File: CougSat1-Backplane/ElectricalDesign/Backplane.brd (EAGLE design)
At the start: 82.8 x 86 mm, 17 parts, among them J1 CougSat Socket, J10 CougSat Socket, J2 CougSat Socket, J3 CougSat Socket, J4 CougSat Socket, J5 Separation Switch, J6 Separation Switch, J7 CougSat Socket, J8 CougSat Socket, J9 CougSat Socket

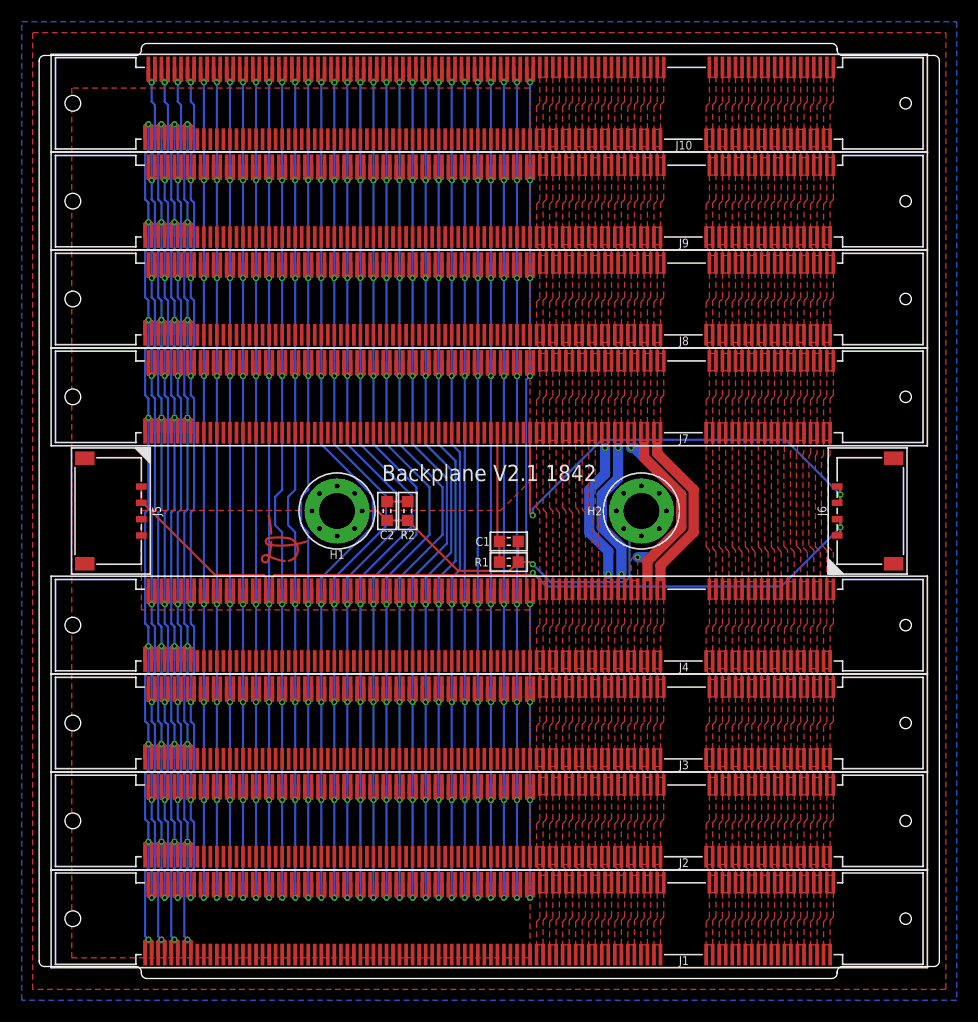
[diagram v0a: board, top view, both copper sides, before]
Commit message: Merge branch 'master' into panel+X
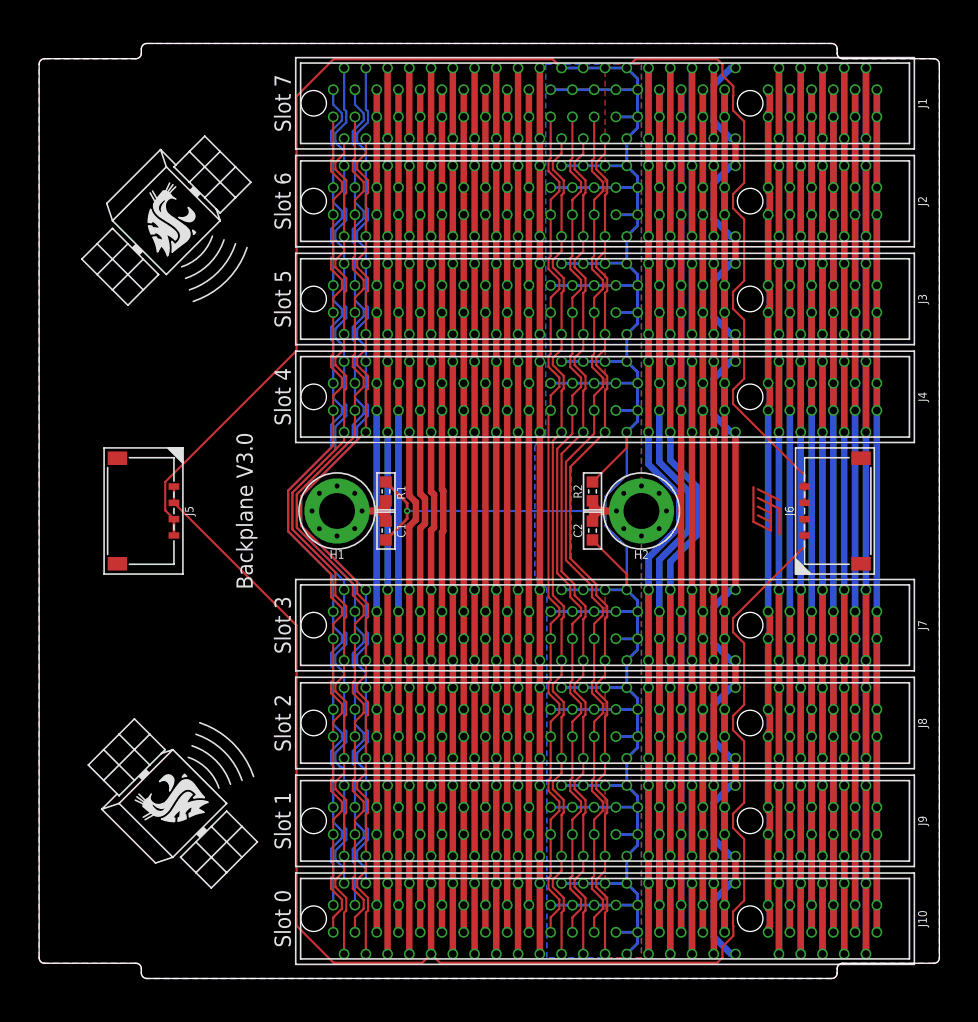
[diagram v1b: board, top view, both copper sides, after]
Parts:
- added LOGO100, LOGO3: Satellite 16mm, CougsInSpace-Aesthetics:CIS-SATELLITE-16
- added LOGO2: SIGNATUREHENDRIK, CougsInSpace-Aesthetics:SIGN-HENDRIK
- J1, J10, J2, J3, J4, J7, J8, J9: device CougsInSpace-Connectors:SODIMM-DDR1 -> CougsInSpace-Connectors:PCIE-8
- LOGO1: value SIGNATUREBRADLEY -> Text; device CougsInSpace-Aesthetics:SIGN-BRADLEY -> CougsInSpace-Aesthetics:CIS-TEXT
- moved J1 78.7 mm to (24.0, 37.5)
- moved J10 78.7 mm to (24.0, -37.5)
- moved J2 61.8 mm to (24.0, 28.5)
- moved J9 61.8 mm to (24.0, -28.5)
- moved J3 45.8 mm to (24.0, 19.5)
- moved J8 45.8 mm to (24.0, -19.5)
- moved J4 31.9 mm to (24.0, 10.5)
- moved J7 31.9 mm to (24.0, -10.5)
- moved C2 19.0 mm to (9.50, -1.80), turned to 270 degrees
- moved R2 17.1 mm to (9.50, 1.80)
- moved R1 13.0 mm to (-9.50, 1.80), turned to 270 degrees
- moved C1 11.3 mm to (-9.50, -1.80), turned to 270 degrees
- moved LOGO1 9.97 mm to (-28.4, 0.10), flipped to the bottom, turned to 90 degrees
- moved J5 3.00 mm to (-29.0, 0.00)
- moved J6 3.00 mm to (29.0, 0.00)
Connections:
- removed net CHASSIS: C1.1, C2.1, H1.1, H1.V1, H1.V2, H1.V3, H1.V4, H1.V5, H1.V6, H1.V7, H1.V8, H2.1, H2.V1, H2.V2, H2.V3, H2.V4, H2.V5, H2.V6, H2.V7, H2.V8, R1.2, R2.2
- removed net GPIO-6: J1.105, J1.107, J10.105, J10.107, J2.105, J2.107, J3.105, J3.107, J4.105, J4.107, J7.105, J7.107, J8.105, J8.107, J9.105, J9.107
- removed net GPIO-7: J1.109, J1.111, J10.109, J10.111, J2.109, J2.111, J3.109, J3.111, J4.109, J4.111, J7.109, J7.111, J8.109, J8.111, J9.109, J9.111
- removed net GPIO-8: J1.113, J1.115, J10.113, J10.115, J2.113, J2.115, J3.113, J3.115, J4.113, J4.115, J7.113, J7.115, J8.113, J8.115, J9.113, J9.115
- removed net GPIO-9: J1.117, J1.119, J10.117, J10.119, J2.117, J2.119, J3.117, J3.119, J4.117, J4.119, J7.117, J7.119, J8.117, J8.119, J9.117, J9.119
- new net CHASSIS1: C1.1, H1.1, H1.V1, H1.V2, H1.V3, H1.V4, H1.V5, H1.V6, H1.V7, H1.V8, R1.2
- new net CHASSIS2: C2.1, H2.1, H2.V1, H2.V2, H2.V3, H2.V4, H2.V5, H2.V6, H2.V7, H2.V8, R2.2
- net BUS_I2C0_IRQ: now also J1.A45, J1.B45, J10.A45, J10.B45, J2.A45, J2.B45, J3.A45, J3.B45, J4.A45, J4.B45, J7.A45, J7.B45, J8.A45, J8.B45, J9.A45, J9.B45; no longer J1.181, J1.183, J10.181, J10.183, J2.181, J2.183, J3.181, J3.183, J4.181, J4.183, J7.181, J7.183, J8.181, J8.183, J9.181, J9.183
- net BUS_I2C0_SCL: now also J1.A44, J1.B44, J10.A44, J10.B44, J2.A44, J2.B44, J3.A44, J3.B44, J4.A44, J4.B44, J7.A44, J7.B44, J8.A44, J8.B44, J9.A44, J9.B44; no longer J1.177, J1.179, J10.177, J10.179, J2.177, J2.179, J3.177, J3.179, J4.177, J4.179, J7.177, J7.179, J8.177, J8.179, J9.177, J9.179
- net BUS_I2C0_SDA: now also J1.A43, J1.B43, J10.A43, J10.B43, J2.A43, J2.B43, J3.A43, J3.B43, J4.A43, J4.B43, J7.A43, J7.B43, J8.A43, J8.B43, J9.A43, J9.B43; no longer J1.173, J1.175, J10.173, J10.175, J2.173, J2.175, J3.173, J3.175, J4.173, J4.175, J7.173, J7.175, J8.173, J8.175, J9.173, J9.175
- net BUS_I2C1_IRQ: now also J1.A32, J1.B32, J10.A32, J10.B32, J2.A32, J2.B32, J3.A32, J3.B32, J4.A32, J4.B32, J7.A32, J7.B32, J8.A32, J8.B32, J9.A32, J9.B32; no longer J1.129, J1.131, J10.129, J10.131, J2.129, J2.131, J3.129, J3.131, J4.129, J4.131, J7.129, J7.131, J8.129, J8.131, J9.129, J9.131
- net BUS_I2C1_SCL: now also J1.A31, J1.B31, J10.A31, J10.B31, J2.A31, J2.B31, J3.A31, J3.B31, J4.A31, J4.B31, J7.A31, J7.B31, J8.A31, J8.B31, J9.A31, J9.B31; no longer J1.125, J1.127, J10.125, J10.127, J2.125, J2.127, J3.125, J3.127, J4.125, J4.127, J7.125, J7.127, J8.125, J8.127, J9.125, J9.127
- net BUS_I2C1_SDA: now also J1.A30, J1.B30, J10.A30, J10.B30, J2.A30, J2.B30, J3.A30, J3.B30, J4.A30, J4.B30, J7.A30, J7.B30, J8.A30, J8.B30, J9.A30, J9.B30; no longer J1.121, J1.123, J10.121, J10.123, J2.121, J2.123, J3.121, J3.123, J4.121, J4.123, J7.121, J7.123, J8.121, J8.123, J9.121, J9.123
- net BUS_JTAG_EN-0: now also J1.B46, J10.B46, J2.B46, J3.B46, J4.B46, J7.B46, J8.B46, J9.B46; no longer J1.186, J1.188, J10.186, J10.188, J2.186, J2.188, J3.186, J3.188, J4.186, J4.188, J7.186, J7.188, J8.186, J8.188, J9.186, J9.188
- net BUS_JTAG_EN-1: now also J1.B47, J10.B47, J2.B47, J3.B47, J4.B47, J7.B47, J8.B47, J9.B47; no longer J1.190, J1.192, J10.190, J10.192, J2.190, J2.192, J3.190, J3.192, J4.190, J4.192, J7.190, J7.192, J8.190, J8.192, J9.190, J9.192
- net BUS_JTAG_EN-2: now also J1.B48, J10.B48, J2.B48, J3.B48, J4.B48, J7.B48, J8.B48, J9.B48; no longer J1.194, J1.196, J10.194, J10.196, J2.194, J2.196, J3.194, J3.196, J4.194, J4.196, J7.194, J7.196, J8.194, J8.196, J9.194, J9.196
- net BUS_JTAG_EN-3: now also J1.B49, J10.B49, J2.B49, J3.B49, J4.B49, J7.B49, J8.B49, J9.B49; no longer J1.198, J1.200, J10.198, J10.200, J2.198, J2.200, J3.198, J3.200, J4.198, J4.200, J7.198, J7.200, J8.198, J8.200, J9.198, J9.200
- net BUS_JTAG_TCK: now also J1.A46, J10.A46, J2.A46, J3.A46, J4.A46, J7.A46, J8.A46, J9.A46; no longer J1.185, J1.187, J10.185, J10.187, J2.185, J2.187, J3.185, J3.187, J4.185, J4.187, J7.185, J7.187, J8.185, J8.187, J9.185, J9.187
- net BUS_JTAG_TDI: now also J1.A47, J10.A47, J2.A47, J3.A47, J4.A47, J7.A47, J8.A47, J9.A47; no longer J1.189, J1.191, J10.189, J10.191, J2.189, J2.191, J3.189, J3.191, J4.189, J4.191, J7.189, J7.191, J8.189, J8.191, J9.189, J9.191
- net BUS_JTAG_TDO: now also J1.A48, J10.A48, J2.A48, J3.A48, J4.A48, J7.A48, J8.A48, J9.A48; no longer J1.193, J1.195, J10.193, J10.195, J2.193, J2.195, J3.193, J3.195, J4.193, J4.195, J7.193, J7.195, J8.193, J8.195, J9.193, J9.195
- net BUS_JTAG_TMS: now also J1.A49, J10.A49, J2.A49, J3.A49, J4.A49, J7.A49, J8.A49, J9.A49; no longer J1.197, J1.199, J10.197, J10.199, J2.197, J2.199, J3.197, J3.199, J4.197, J4.199, J7.197, J7.199, J8.197, J8.199, J9.197, J9.199
- net BUS_SPI_MISO: now also J1.A38, J1.B38, J10.A38, J10.B38, J2.A38, J2.B38, J3.A38, J3.B38, J4.A38, J4.B38, J7.A38, J7.B38, J8.A38, J8.B38, J9.A38, J9.B38; no longer J1.153, J1.155, J10.153, J10.155, J2.153, J2.155, J3.153, J3.155, J4.153, J4.155, J7.153, J7.155, J8.153, J8.155, J9.153, J9.155
- net BUS_SPI_MOSI: now also J1.A39, J1.B39, J10.A39, J10.B39, J2.A39, J2.B39, J3.A39, J3.B39, J4.A39, J4.B39, J7.A39, J7.B39, J8.A39, J8.B39, J9.A39, J9.B39; no longer J1.157, J1.159, J10.157, J10.159, J2.157, J2.159, J3.157, J3.159, J4.157, J4.159, J7.157, J7.159, J8.157, J8.159, J9.157, J9.159
- net BUS_SPI_SCK: now also J1.A37, J1.B37, J10.A37, J10.B37, J2.A37, J2.B37, J3.A37, J3.B37, J4.A37, J4.B37, J7.A37, J7.B37, J8.A37, J8.B37, J9.A37, J9.B37; no longer J1.149, J1.151, J10.149, J10.151, J2.149, J2.151, J3.149, J3.151, J4.149, J4.151, J7.149, J7.151, J8.149, J8.151, J9.149, J9.151
- net COM_SPI_CS: now also J1.A36, J1.B36, J10.A36, J10.B36, J2.A36, J2.B36, J3.A36, J3.B36, J4.A36, J4.B36, J7.A36, J7.B36, J8.A36, J8.B36, J9.A36, J9.B36; no longer J1.145, J1.147, J10.145, J10.147, J2.145, J2.147, J3.145, J3.147, J4.145, J4.147, J7.145, J7.147, J8.145, J8.147, J9.145, J9.147
- net COM_SPI_MISO: now also J1.A34, J1.B34, J10.A34, J10.B34, J2.A34, J2.B34, J3.A34, J3.B34, J4.A34, J4.B34, J7.A34, J7.B34, J8.A34, J8.B34, J9.A34, J9.B34; no longer J1.137, J1.139, J10.137, J10.139, J2.137, J2.139, J3.137, J3.139, J4.137, J4.139, J7.137, J7.139, J8.137, J8.139, J9.137, J9.139
- net COM_SPI_MOSI: now also J1.A35, J1.B35, J10.A35, J10.B35, J2.A35, J2.B35, J3.A35, J3.B35, J4.A35, J4.B35, J7.A35, J7.B35, J8.A35, J8.B35, J9.A35, J9.B35; no longer J1.141, J1.143, J10.141, J10.143, J2.141, J2.143, J3.141, J3.143, J4.141, J4.143, J7.141, J7.143, J8.141, J8.143, J9.141, J9.143
- net COM_SPI_SCK: now also J1.A33, J1.B33, J10.A33, J10.B33, J2.A33, J2.B33, J3.A33, J3.B33, J4.A33, J4.B33, J7.A33, J7.B33, J8.A33, J8.B33, J9.A33, J9.B33; no longer J1.133, J1.135, J10.133, J10.135, J2.133, J2.135, J3.133, J3.135, J4.133, J4.135, J7.133, J7.135, J8.133, J8.135, J9.133, J9.135
- net CTRL_!RESET: now also J1.A41, J1.B41, J10.A41, J10.B41, J2.A41, J2.B41, J3.A41, J3.B41, J4.A41, J4.B41, J7.A41, J7.B41, J8.A41, J8.B41, J9.A41, J9.B41; no longer J1.165, J1.167, J10.165, J10.167, J2.165, J2.167, J3.165, J3.167, J4.165, J4.167, J7.165, J7.167, J8.165, J8.167, J9.165, J9.167
- net CTRL_SYNC: now also J1.A42, J1.B42, J10.A42, J10.B42, J2.A42, J2.B42, J3.A42, J3.B42, J4.A42, J4.B42, J7.A42, J7.B42, J8.A42, J8.B42, J9.A42, J9.B42; no longer J1.169, J1.171, J10.169, J10.171, J2.169, J2.171, J3.169, J3.171, J4.169, J4.171, J7.169, J7.171, J8.169, J8.171, J9.169, J9.171
- net GPIO-0: now also J1.A24, J10.A24, J2.A24, J3.A24, J4.A24, J7.A24, J8.A24, J9.A24; no longer J1.81, J1.83, J10.81, J10.83, J2.81, J2.83, J3.81, J3.83, J4.81, J4.83, J7.81, J7.83, J8.81, J8.83, J9.81, J9.83
- net GPIO-1: now also J1.A25, J10.A25, J2.A25, J3.A25, J4.A25, J7.A25, J8.A25, J9.A25; no longer J1.85, J1.87, J10.85, J10.87, J2.85, J2.87, J3.85, J3.87, J4.85, J4.87, J7.85, J7.87, J8.85, J8.87, J9.85, J9.87
- net GPIO-2: now also J1.A26, J10.A26, J2.A26, J3.A26, J4.A26, J7.A26, J8.A26, J9.A26; no longer J1.89, J1.91, J10.89, J10.91, J2.89, J2.91, J3.89, J3.91, J4.89, J4.91, J7.89, J7.91, J8.89, J8.91, J9.89, J9.91
- net GPIO-3: now also J1.A27, J10.A27, J2.A27, J3.A27, J4.A27, J7.A27, J8.A27, J9.A27; no longer J1.93, J1.95, J10.93, J10.95, J2.93, J2.95, J3.93, J3.95, J4.93, J4.95, J7.93, J7.95, J8.93, J8.95, J9.93, J9.95
- net GPIO-4: now also J1.A28, J10.A28, J2.A28, J3.A28, J4.A28, J7.A28, J8.A28, J9.A28; no longer J1.97, J1.99, J10.97, J10.99, J2.97, J2.99, J3.97, J3.99, J4.97, J4.99, J7.97, J7.99, J8.97, J8.99, J9.97, J9.99
- net GPIO-5: now also J1.A29, J10.A29, J2.A29, J3.A29, J4.A29, J7.A29, J8.A29, J9.A29; no longer J1.101, J1.103, J10.101, J10.103, J2.101, J2.103, J3.101, J3.103, J4.101, J4.103, J7.101, J7.103, J8.101, J8.103, J9.101, J9.103
- net PGND: now also J1.A21, J1.A22, J1.A23, J1.B21, J1.B22, J1.B23, J1.B24, J1.B25, J1.B26, J1.B27, J1.B28, J1.B29, J10.A21, J10.A22, J10.A23, J10.B21, J10.B22, J10.B23, J10.B24, J10.B25, J10.B26, J10.B27, J10.B28, J10.B29, J2.A21, J2.A22, J2.A23, J2.B21, J2.B22, J2.B23, J2.B24, J2.B25, J2.B26, J2.B27, J2.B28, J2.B29, J3.A21, J3.A22, J3.A23, J3.B21, J3.B22, J3.B23, J3.B24, J3.B25, J3.B26, J3.B27, J3.B28, J3.B29, J4.A21, J4.A22, J4.A23, J4.B21, J4.B22, J4.B23, J4.B24, J4.B25, J4.B26, J4.B27, J4.B28, J4.B29, J7.A21, J7.A22, J7.A23, J7.B21, J7.B22, J7.B23, J7.B24, J7.B25, J7.B26, J7.B27, J7.B28, J7.B29, J8.A21, J8.A22, J8.A23, J8.B21, J8.B22, J8.B23, J8.B24, J8.B25, J8.B26, J8.B27, J8.B28, J8.B29, J9.A21, J9.A22, J9.A23, J9.B21, J9.B22, J9.B23, J9.B24, J9.B25, J9.B26, J9.B27, J9.B28, J9.B29; no longer J1.100, J1.102, J1.104, J1.106, J1.108, J1.110, J1.112, J1.114, J1.116, J1.118, J1.120, J1.122, J1.124, J1.126, J1.128, J1.130, J1.132, J1.134, J1.136, J1.138, J1.140, J1.142, J1.144, J1.146, J1.148, J1.150, J1.152, J1.154, J1.156, J1.158, J1.160, J1.162, J1.164, J1.166, J1.168, J1.170, J1.172, J1.174, J1.176, J1.178, J1.180, J1.182, J1.184, J1.82, J1.84, J1.86, J1.88, J1.90, J1.92, J1.94, J1.96, J1.98, J10.100, J10.102, J10.104, J10.106, J10.108, J10.110, J10.112, J10.114, J10.116, J10.118, J10.120, J10.122, J10.124, J10.126, J10.128, J10.130, J10.132, J10.134, J10.136, J10.138, J10.140, J10.142, J10.144, J10.146, J10.148, J10.150, J10.152, J10.154, J10.156, J10.158, J10.160, J10.162, J10.164, J10.166, J10.168, J10.170, J10.172, J10.174, J10.176, J10.178, J10.180, J10.182, J10.184, J10.82, J10.84, J10.86, J10.88, J10.90, J10.92, J10.94, J10.96, J10.98, J2.100, J2.102, J2.104, J2.106, J2.108, J2.110, J2.112, J2.114, J2.116, J2.118, J2.120, J2.122, J2.124, J2.126, J2.128, J2.130, J2.132, J2.134, J2.136, J2.138, J2.140, J2.142, J2.144, J2.146, J2.148, J2.150, J2.152, J2.154, J2.156, J2.158, J2.160, J2.162, J2.164, J2.166, J2.168, J2.170, J2.172, J2.174, J2.176, J2.178, J2.180, J2.182, J2.184, J2.82, J2.84, J2.86, J2.88, J2.90, J2.92, J2.94, J2.96, J2.98, J3.100, J3.102, J3.104, J3.106, J3.108, J3.110, J3.112, J3.114, J3.116, J3.118, J3.120, J3.122, J3.124, J3.126, J3.128, J3.130, J3.132, J3.134, J3.136, J3.138, J3.140, J3.142, J3.144, J3.146, J3.148, J3.150, J3.152, J3.154, J3.156, J3.158, J3.160, J3.162, J3.164, J3.166, J3.168, J3.170, J3.172, J3.174, J3.176, J3.178, J3.180, J3.182, J3.184, J3.82, J3.84, J3.86, J3.88, J3.90, J3.92, J3.94, J3.96, J3.98, J4.100, J4.102, J4.104, J4.106, J4.108, J4.110, J4.112, J4.114, J4.116, J4.118, J4.120, J4.122, J4.124, J4.126, J4.128, J4.130, J4.132, J4.134, J4.136, J4.138, J4.140, J4.142, J4.144, J4.146, J4.148, J4.150, J4.152, J4.154, J4.156, J4.158, J4.160, J4.162, J4.164, J4.166, J4.168, J4.170, J4.172, J4.174, J4.176, J4.178, J4.180, J4.182, J4.184, J4.82, J4.84, J4.86, J4.88, J4.90, J4.92, J4.94, J4.96, J4.98, J7.100, J7.102, J7.104, J7.106, J7.108, J7.110, J7.112, J7.114, J7.116, J7.118, J7.120, J7.122, J7.124, J7.126, J7.128, J7.130, J7.132, J7.134, J7.136, J7.138, J7.140, J7.142, J7.144, J7.146, J7.148, J7.150, J7.152, J7.154, J7.156, J7.158, J7.160, J7.162, J7.164, J7.166, J7.168, J7.170, J7.172, J7.174, J7.176, J7.178, J7.180, J7.182, J7.184, J7.82, J7.84, J7.86, J7.88, J7.90, J7.92, J7.94, J7.96, J7.98, J8.100, J8.102, J8.104, J8.106, J8.108, J8.110, J8.112, J8.114, J8.116, J8.118, J8.120, J8.122, J8.124, J8.126, J8.128, J8.130, J8.132, J8.134, J8.136, J8.138, J8.140, J8.142, J8.144, J8.146, J8.148, J8.150, J8.152, J8.154, J8.156, J8.158, J8.160, J8.162, J8.164, J8.166, J8.168, J8.170, J8.172, J8.174, J8.176, J8.178, J8.180, J8.182, J8.184, J8.82, J8.84, J8.86, J8.88, J8.90, J8.92, J8.94, J8.96, J8.98, J9.100, J9.102, J9.104, J9.106, J9.108, J9.110, J9.112, J9.114, J9.116, J9.118, J9.120, J9.122, J9.124, J9.126, J9.128, J9.130, J9.132, J9.134, J9.136, J9.138, J9.140, J9.142, J9.144, J9.146, J9.148, J9.150, J9.152, J9.154, J9.156, J9.158, J9.160, J9.162, J9.164, J9.166, J9.168, J9.170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
- net PR_3.3V-0: now also J1.A1, J1.B1, J10.A1, J10.B1, J2.A1, J2.B1, J3.A1, J3.B1, J4.A1, J4.B1, J7.A1, J7.B1, J8.A1, J8.B1, J9.A1, J9.B1; no longer J1.1, J1.2, J1.3, J1.4, J10.1, J10.2, J10.3, J10.4, J2.1, J2.2, J2.3, J2.4, J3.1, J3.2, J3.3, J3.4, J4.1, J4.2, J4.3, J4.4, J7.1, J7.2, J7.3, J7.4, J8.1, J8.2, J8.3, J8.4, J9.1, J9.2, J9.3, J9.4
- net PR_3.3V-1: now also J1.A2, J1.B2, J10.A2, J10.B2, J2.A2, J2.B2, J3.A2, J3.B2, J4.A2, J4.B2, J7.A2, J7.B2, J8.A2, J8.B2, J9.A2, J9.B2; no longer J1.5, J1.6, J1.7, J1.8, J10.5, J10.6, J10.7, J10.8, J2.5, J2.6, J2.7, J2.8, J3.5, J3.6, J3.7, J3.8, J4.5, J4.6, J4.7, J4.8, J7.5, J7.6, J7.7, J7.8, J8.5, J8.6, J8.7, J8.8, J9.5, J9.6, J9.7, J9.8
- net PR_3.3V-10: now also J1.A11, J1.B11, J10.A11, J10.B11, J2.A11, J2.B11, J3.A11, J3.B11, J4.A11, J4.B11, J7.A11, J7.B11, J8.A11, J8.B11, J9.A11, J9.B11; no longer J1.41, J1.42, J1.43, J1.44, J10.41, J10.42, J10.43, J10.44, J2.41, J2.42, J2.43, J2.44, J3.41, J3.42, J3.43, J3.44, J4.41, J4.42, J4.43, J4.44, J7.41, J7.42, J7.43, J7.44, J8.41, J8.42, J8.43, J8.44, J9.41, J9.42, J9.43, J9.44
- net PR_3.3V-11: now also J1.A12, J1.B12, J10.A12, J10.B12, J2.A12, J2.B12, J3.A12, J3.B12, J4.A12, J4.B12, J7.A12, J7.B12, J8.A12, J8.B12, J9.A12, J9.B12; no longer J1.45, J1.46, J1.47, J1.48, J10.45, J10.46, J10.47, J10.48, J2.45, J2.46, J2.47, J2.48, J3.45, J3.46, J3.47, J3.48, J4.45, J4.46, J4.47, J4.48, J7.45, J7.46, J7.47, J7.48, J8.45, J8.46, J8.47, J8.48, J9.45, J9.46, J9.47, J9.48
- net PR_3.3V-12: now also J1.A13, J1.B13, J10.A13, J10.B13, J2.A13, J2.B13, J3.A13, J3.B13, J4.A13, J4.B13, J7.A13, J7.B13, J8.A13, J8.B13, J9.A13, J9.B13; no longer J1.49, J1.50, J1.51, J1.52, J10.49, J10.50, J10.51, J10.52, J2.49, J2.50, J2.51, J2.52, J3.49, J3.50, J3.51, J3.52, J4.49, J4.50, J4.51, J4.52, J7.49, J7.50, J7.51, J7.52, J8.49, J8.50, J8.51, J8.52, J9.49, J9.50, J9.51, J9.52
- net PR_3.3V-2: now also J1.A3, J1.B3, J10.A3, J10.B3, J2.A3, J2.B3, J3.A3, J3.B3, J4.A3, J4.B3, J7.A3, J7.B3, J8.A3, J8.B3, J9.A3, J9.B3; no longer J1.10, J1.11, J1.12, J1.9, J10.10, J10.11, J10.12, J10.9, J2.10, J2.11, J2.12, J2.9, J3.10, J3.11, J3.12, J3.9, J4.10, J4.11, J4.12, J4.9, J7.10, J7.11, J7.12, J7.9, J8.10, J8.11, J8.12, J8.9, J9.10, J9.11, J9.12, J9.9
- net PR_3.3V-3: now also J1.A4, J1.B4, J10.A4, J10.B4, J2.A4, J2.B4, J3.A4, J3.B4, J4.A4, J4.B4, J7.A4, J7.B4, J8.A4, J8.B4, J9.A4, J9.B4; no longer J1.13, J1.14, J1.15, J1.16, J10.13, J10.14, J10.15, J10.16, J2.13, J2.14, J2.15, J2.16, J3.13, J3.14, J3.15, J3.16, J4.13, J4.14, J4.15, J4.16, J7.13, J7.14, J7.15, J7.16, J8.13, J8.14, J8.15, J8.16, J9.13, J9.14, J9.15, J9.16
- net PR_3.3V-4: now also J1.A5, J1.B5, J10.A5, J10.B5, J2.A5, J2.B5, J3.A5, J3.B5, J4.A5, J4.B5, J7.A5, J7.B5, J8.A5, J8.B5, J9.A5, J9.B5; no longer J1.17, J1.18, J1.19, J1.20, J10.17, J10.18, J10.19, J10.20, J2.17, J2.18, J2.19, J2.20, J3.17, J3.18, J3.19, J3.20, J4.17, J4.18, J4.19, J4.20, J7.17, J7.18, J7.19, J7.20, J8.17, J8.18, J8.19, J8.20, J9.17, J9.18, J9.19, J9.20
- net PR_3.3V-5: now also J1.A6, J1.B6, J10.A6, J10.B6, J2.A6, J2.B6, J3.A6, J3.B6, J4.A6, J4.B6, J7.A6, J7.B6, J8.A6, J8.B6, J9.A6, J9.B6; no longer J1.21, J1.22, J1.23, J1.24, J10.21, J10.22, J10.23, J10.24, J2.21, J2.22, J2.23, J2.24, J3.21, J3.22, J3.23, J3.24, J4.21, J4.22, J4.23, J4.24, J7.21, J7.22, J7.23, J7.24, J8.21, J8.22, J8.23, J8.24, J9.21, J9.22, J9.23, J9.24
- net PR_3.3V-6: now also J1.A7, J1.B7, J10.A7, J10.B7, J2.A7, J2.B7, J3.A7, J3.B7, J4.A7, J4.B7, J7.A7, J7.B7, J8.A7, J8.B7, J9.A7, J9.B7; no longer J1.25, J1.26, J1.27, J1.28, J10.25, J10.26, J10.27, J10.28, J2.25, J2.26, J2.27, J2.28, J3.25, J3.26, J3.27, J3.28, J4.25, J4.26, J4.27, J4.28, J7.25, J7.26, J7.27, J7.28, J8.25, J8.26, J8.27, J8.28, J9.25, J9.26, J9.27, J9.28
- net PR_3.3V-7: now also J1.A8, J1.B8, J10.A8, J10.B8, J2.A8, J2.B8, J3.A8, J3.B8, J4.A8, J4.B8, J7.A8, J7.B8, J8.A8, J8.B8, J9.A8, J9.B8; no longer J1.29, J1.30, J1.31, J1.32, J10.29, J10.30, J10.31, J10.32, J2.29, J2.30, J2.31, J2.32, J3.29, J3.30, J3.31, J3.32, J4.29, J4.30, J4.31, J4.32, J7.29, J7.30, J7.31, J7.32, J8.29, J8.30, J8.31, J8.32, J9.29, J9.30, J9.31, J9.32
- net PR_3.3V-8: now also J1.A9, J1.B9, J10.A9, J10.B9, J2.A9, J2.B9, J3.A9, J3.B9, J4.A9, J4.B9, J7.A9, J7.B9, J8.A9, J8.B9, J9.A9, J9.B9; no longer J1.33, J1.34, J1.35, J1.36, J10.33, J10.34, J10.35, J10.36, J2.33, J2.34, J2.35, J2.36, J3.33, J3.34, J3.35, J3.36, J4.33, J4.34, J4.35, J4.36, J7.33, J7.34, J7.35, J7.36, J8.33, J8.34, J8.35, J8.36, J9.33, J9.34, J9.35, J9.36
- net PR_3.3V-9: now also J1.A10, J1.B10, J10.A10, J10.B10, J2.A10, J2.B10, J3.A10, J3.B10, J4.A10, J4.B10, J7.A10, J7.B10, J8.A10, J8.B10, J9.A10, J9.B10; no longer J1.37, J1.38, J1.39, J1.40, J10.37, J10.38, J10.39, J10.40, J2.37, J2.38, J2.39, J2.40, J3.37, J3.38, J3.39, J3.40, J4.37, J4.38, J4.39, J4.40, J7.37, J7.38, J7.39, J7.40, J8.37, J8.38, J8.39, J8.40, J9.37, J9.38, J9.39, J9.40
- net PR_BATT-0: now also J1.A14, J1.B14, J10.A14, J10.B14, J2.A14, J2.B14, J3.A14, J3.B14, J4.A14, J4.B14, J7.A14, J7.B14, J8.A14, J8.B14, J9.A14, J9.B14; no longer J1.53, J1.54, J1.55, J1.56, J10.53, J10.54, J10.55, J10.56, J2.53, J2.54, J2.55, J2.56, J3.53, J3.54, J3.55, J3.56, J4.53, J4.54, J4.55, J4.56, J7.53, J7.54, J7.55, J7.56, J8.53, J8.54, J8.55, J8.56, J9.53, J9.54, J9.55, J9.56
- net PR_BATT-1: now also J1.A15, J1.B15, J10.A15, J10.B15, J2.A15, J2.B15, J3.A15, J3.B15, J4.A15, J4.B15, J7.A15, J7.B15, J8.A15, J8.B15, J9.A15, J9.B15; no longer J1.57, J1.58, J1.59, J1.60, J10.57, J10.58, J10.59, J10.60, J2.57, J2.58, J2.59, J2.60, J3.57, J3.58, J3.59, J3.60, J4.57, J4.58, J4.59, J4.60, J7.57, J7.58, J7.59, J7.60, J8.57, J8.58, J8.59, J8.60, J9.57, J9.58, J9.59, J9.60
- net PR_BATT-2: now also J1.A16, J1.B16, J10.A16, J10.B16, J2.A16, J2.B16, J3.A16, J3.B16, J4.A16, J4.B16, J7.A16, J7.B16, J8.A16, J8.B16, J9.A16, J9.B16; no longer J1.61, J1.62, J1.63, J1.64, J10.61, J10.62, J10.63, J10.64, J2.61, J2.62, J2.63, J2.64, J3.61, J3.62, J3.63, J3.64, J4.61, J4.62, J4.63, J4.64, J7.61, J7.62, J7.63, J7.64, J8.61, J8.62, J8.63, J8.64, J9.61, J9.62, J9.63, J9.64
- net PR_BATT-3: now also J1.A17, J1.B17, J10.A17, J10.B17, J2.A17, J2.B17, J3.A17, J3.B17, J4.A17, J4.B17, J7.A17, J7.B17, J8.A17, J8.B17, J9.A17, J9.B17; no longer J1.65, J1.66, J1.67, J1.68, J10.65, J10.66, J10.67, J10.68, J2.65, J2.66, J2.67, J2.68, J3.65, J3.66, J3.67, J3.68, J4.65, J4.66, J4.67, J4.68, J7.65, J7.66, J7.67, J7.68, J8.65, J8.66, J8.67, J8.68, J9.65, J9.66, J9.67, J9.68
- net PR_BATT-4: now also J1.A18, J1.B18, J10.A18, J10.B18, J2.A18, J2.B18, J3.A18, J3.B18, J4.A18, J4.B18, J7.A18, J7.B18, J8.A18, J8.B18, J9.A18, J9.B18; no longer J1.69, J1.70, J1.71, J1.72, J10.69, J10.70, J10.71, J10.72, J2.69, J2.70, J2.71, J2.72, J3.69, J3.70, J3.71, J3.72, J4.69, J4.70, J4.71, J4.72, J7.69, J7.70, J7.71, J7.72, J8.69, J8.70, J8.71, J8.72, J9.69, J9.70, J9.71, J9.72
- net PR_BATT-5: now also J1.A19, J1.B19, J10.A19, J10.B19, J2.A19, J2.B19, J3.A19, J3.B19, J4.A19, J4.B19, J7.A19, J7.B19, J8.A19, J8.B19, J9.A19, J9.B19; no longer J1.73, J1.74, J1.75, J1.76, J10.73, J10.74, J10.75, J10.76, J2.73, J2.74, J2.75, J2.76, J3.73, J3.74, J3.75, J3.76, J4.73, J4.74, J4.75, J4.76, J7.73, J7.74, J7.75, J7.76, J8.73, J8.74, J8.75, J8.76, J9.73, J9.74, J9.75, J9.76
- net PR_BATT-6: now also J1.A20, J1.B20, J10.A20, J10.B20, J2.A20, J2.B20, J3.A20, J3.B20, J4.A20, J4.B20, J7.A20, J7.B20, J8.A20, J8.B20, J9.A20, J9.B20; no longer J1.77, J1.78, J1.79, J1.80, J10.77, J10.78, J10.79, J10.80, J2.77, J2.78, J2.79, J2.80, J3.77, J3.78, J3.79, J3.80, J4.77, J4.78, J4.79, J4.80, J7.77, J7.78, J7.79, J7.80, J8.77, J8.78, J8.79, J8.80, J9.77, J9.78, J9.79, J9.80
- net PWR_CTRL_SW: now also J1.A40, J1.B40, J10.A40, J10.B40, J2.A40, J2.B40, J3.A40, J3.B40, J4.A40, J4.B40, J7.A40, J7.B40, J8.A40, J8.B40, J9.A40, J9.B40; no longer J1.161, J1.163, J10.161, J10.163, J2.161, J2.163, J3.161, J3.163, J4.161, J4.163, J7.161, J7.163, J8.161, J8.163, J9.161, J9.163
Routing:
- net PGND: track 57.0 -> 382.0 mm, vias 2 -> 1
- net PR_BATT-2: track 0.00 -> 148.5 mm
- net PR_3.3V-9: track 0.00 -> 148.5 mm
- net PR_3.3V-7: track 0.00 -> 148.5 mm
- net PR_3.3V-5: track 0.00 -> 148.5 mm
- net PR_3.3V-3: track 0.00 -> 148.5 mm
- net PR_3.3V-1: track 0.00 -> 148.5 mm
- net PR_BATT-6: track 0.00 -> 144.4 mm
- net PR_BATT-4: track 0.00 -> 144.1 mm
- net PR_BATT-3: track 0.00 -> 136.5 mm
- net PR_3.3V-8: track 0.00 -> 136.5 mm
- net PR_3.3V-6: track 0.00 -> 136.5 mm
- net PR_3.3V-4: track 0.00 -> 136.5 mm
- net PR_3.3V-2: track 0.00 -> 136.5 mm
- net PR_3.3V-0: track 0.00 -> 136.5 mm
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- added copper zone on layer 16, net BALANCING-TOP
- added copper zone on layer 16, net PGND
- removed copper zone on layer 16, net BALANCING-BOTTOM
- removed copper zone on layer 1, net BUS_I2C0_IRQ
- removed copper zone on layer 1, net BUS_I2C0_SCL
- removed copper zone on layer 1, net BUS_I2C0_SDA
- removed copper zone on layer 1, net BUS_I2C1_IRQ
- removed copper zone on layer 1, net BUS_I2C1_SCL
- removed copper zone on layer 1, net BUS_I2C1_SDA
- removed copper zone on layer 1, net BUS_JTAG_EN-0
- removed copper zone on layer 1, net BUS_JTAG_EN-1
- removed copper zone on layer 1, net BUS_JTAG_EN-2
- removed copper zone on layer 1, net BUS_JTAG_EN-3
- removed copper zone on layer 1, net BUS_JTAG_TCK
- removed copper zone on layer 1, net BUS_JTAG_TDI
- removed copper zone on layer 1, net BUS_JTAG_TDO
- removed copper zone on layer 1, net BUS_JTAG_TMS
- removed copper zone on layer 1, net BUS_SPI_MISO
- removed copper zone on layer 1, net BUS_SPI_MOSI
- removed copper zone on layer 1, net BUS_SPI_SCK
- removed copper zone on layer 1, net COM_SPI_CS
- removed copper zone on layer 1, net COM_SPI_MISO
- removed copper zone on layer 1, net COM_SPI_MOSI
- removed copper zone on layer 1, net COM_SPI_SCK
- removed copper zone on layer 1, net CTRL_!RESET
- removed copper zone on layer 1, net CTRL_SYNC
- removed copper zone on layer 1, net GPIO-0
- removed copper zone on layer 1, net GPIO-1
- removed copper zone on layer 1, net GPIO-2
- removed copper zone on layer 1, net GPIO-3
- removed copper zone on layer 1, net GPIO-4
- removed copper zone on layer 1, net GPIO-5
- removed copper zone on layer 1, net GPIO-6
- removed copper zone on layer 1, net GPIO-7
- removed copper zone on layer 1, net GPIO-8
- removed copper zone on layer 1, net GPIO-9
- removed copper zone on layer 1, net PR_3.3V-0
- removed copper zone on layer 1, net PR_3.3V-1
- removed copper zone on layer 1, net PR_3.3V-10
- removed copper zone on layer 1, net PR_3.3V-11
- removed copper zone on layer 1, net PR_3.3V-12
- removed copper zone on layer 1, net PR_3.3V-2
- removed copper zone on layer 1, net PR_3.3V-3
- removed copper zone on layer 1, net PR_3.3V-4
- removed copper zone on layer 1, net PR_3.3V-5
- removed copper zone on layer 1, net PR_3.3V-6
- removed copper zone on layer 1, net PR_3.3V-7
- removed copper zone on layer 1, net PR_3.3V-8
- removed copper zone on layer 1, net PR_3.3V-9
- removed copper zone on layer 1, net PR_BATT-0
- removed copper zone on layer 1, net PR_BATT-1
- removed copper zone on layer 1, net PR_BATT-2
- removed copper zone on layer 1, net PR_BATT-3
- removed copper zone on layer 1, net PR_BATT-4
- removed copper zone on layer 1, net PR_BATT-5
- removed copper zone on layer 1, net PR_BATT-6
- removed copper zone on layer 1, net PWR_CTRL_SW
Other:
- outline, holes or cut-outs redrawn
- board text added: "Backplane V3.0"
- board text added: "Slot 0"
- board text added: "Slot 1"
- board text added: "Slot 2"
- board text added: "Slot 3"
- board text added: "Slot 4"
- board text added: "Slot 5"
- board text added: "Slot 6"
- board text added: "Slot 7"
- board text removed: "Backplane V2.1 1842"
